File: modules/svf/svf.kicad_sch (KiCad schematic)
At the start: 23 parts, among them U1 MCP6002-xSN, U2 MCP6002-xSN

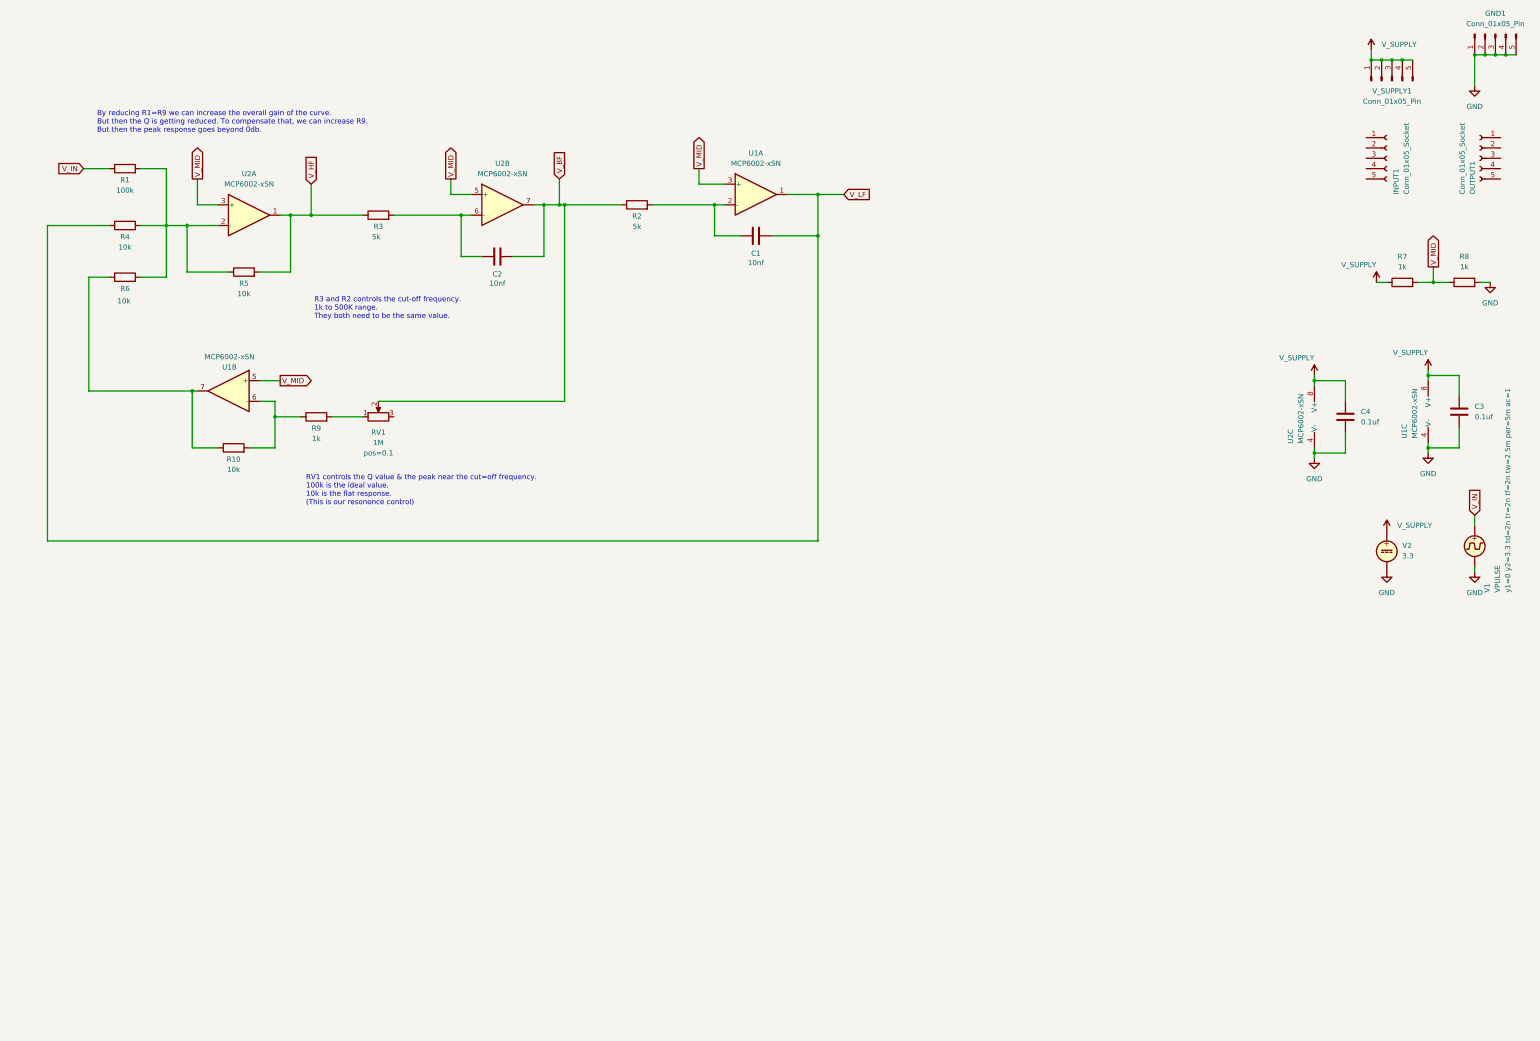
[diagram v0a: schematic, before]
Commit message: Implement the final schematic for SVF
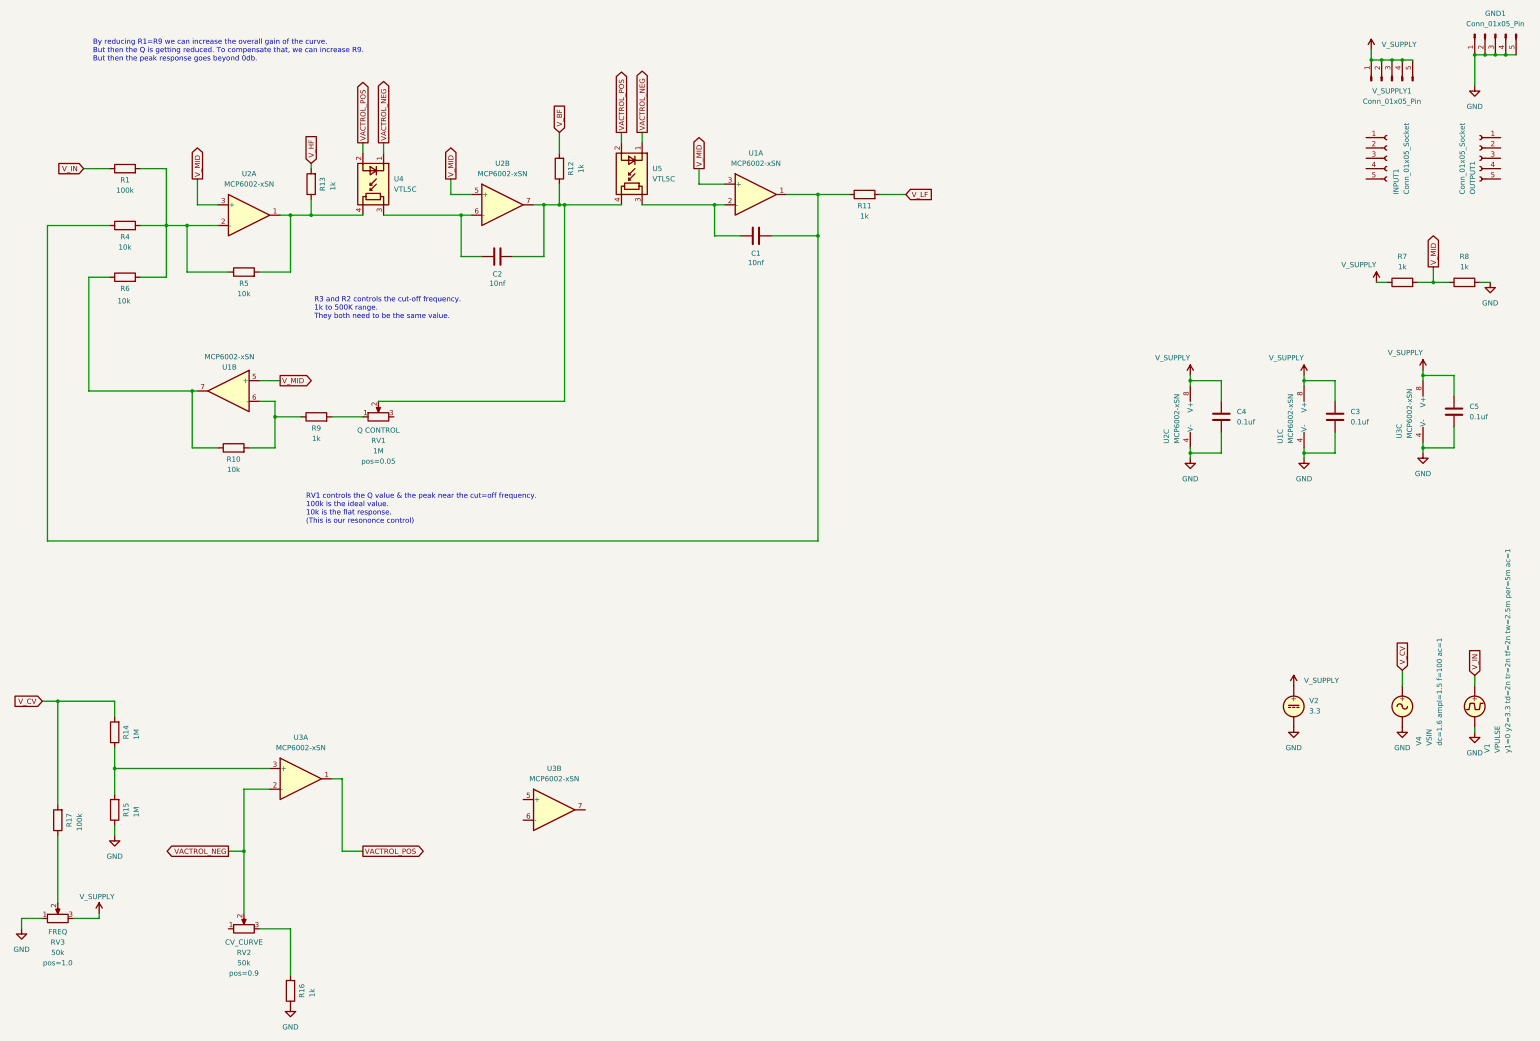
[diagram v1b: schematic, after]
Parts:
- removed R2, R3: 5k, symbol Device:R
- added C5: 0.1uf, symbol Device:C
- added R11, R12, R13, R16: 1k, symbol Device:R
- added R14, R15: 1M, symbol Device:R
- added R17: 100k, symbol Device:R
- added RV2, RV3: 50k, symbol Device:R_Potentiometer
- added U3: MCP6002-xSN, symbol Amplifier_Operational:MCP6002-xSN
- added U4, U5: VTL5C, BreadModular_MISC:VTL5C, symbol Isolator:VTL5C
- added V4: VSIN, symbol Simulation_SPICE:VSIN
- RV1: Comments (none) -> Q CONTROL
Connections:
- net GND: now also C5.2, R15.1, R16.1, RV3.1, U3.4 (V-), V4.2
- net V_BF: now also R12.2; no longer C2.2, RV1.2, U2.7
- net V_HF: now also R13.2; no longer R5.2, U2.1
- net V_LF: now also R11.2; no longer C1.2, R4.1, U1.1
- net V_SUPPLY: now also C5.1, RV3.3, U3.8 (V+)
- net at C1.1, U1.2 (-): now also U5.3
- net at C2.1, U2.6 (-): now also U4.3
- new net: R13.1, R5.2, U2.1, U4.4
- new net: C1.2, R11.1, R4.1, U1.1
- new net: C2.2, R12.1, RV1.2, U2.7, U5.4
- new net: R16.2, RV2.3
- new net: R17.1, RV3.2
- new net: R14.1, R15.2, U3.3 (+)
- new net VACTROL_NEG: RV2.2, U3.2 (-), U4.1 (-), U5.1 (-)
- new net VACTROL_POS: U3.1, U4.2 (+), U5.2 (+)
- new net V_CV: R14.2, R17.2, V4.1
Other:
- moved on the sheet: C3, C4, U1C, U2C, V1, V2
